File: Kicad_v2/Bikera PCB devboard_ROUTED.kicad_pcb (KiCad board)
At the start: 4 copper layers, 60 x 40 mm, 114 parts, among them IC1 DRV5032DULPGM, IC2 BQ25630YBGR, IC3 DRV5032DULPGM, IC4 FM24V01A-G, J1 USB4105-GF-A-060, J3 ST-LINK BTB, J7 Waveshare_ePaper_module, SW1 SW_Reset, SW2 SW_Boot, U1 RT6158HWSC, U2 TCR3UG33A_LF, U3 STM32L431CCTx, U4 TPS61253F, U5 ATECC608B-SSHDA-T, U6 LC76GPAMD, U7 USBLC6-2SC6, U8 SMF05CT1G, U9 RAK11720

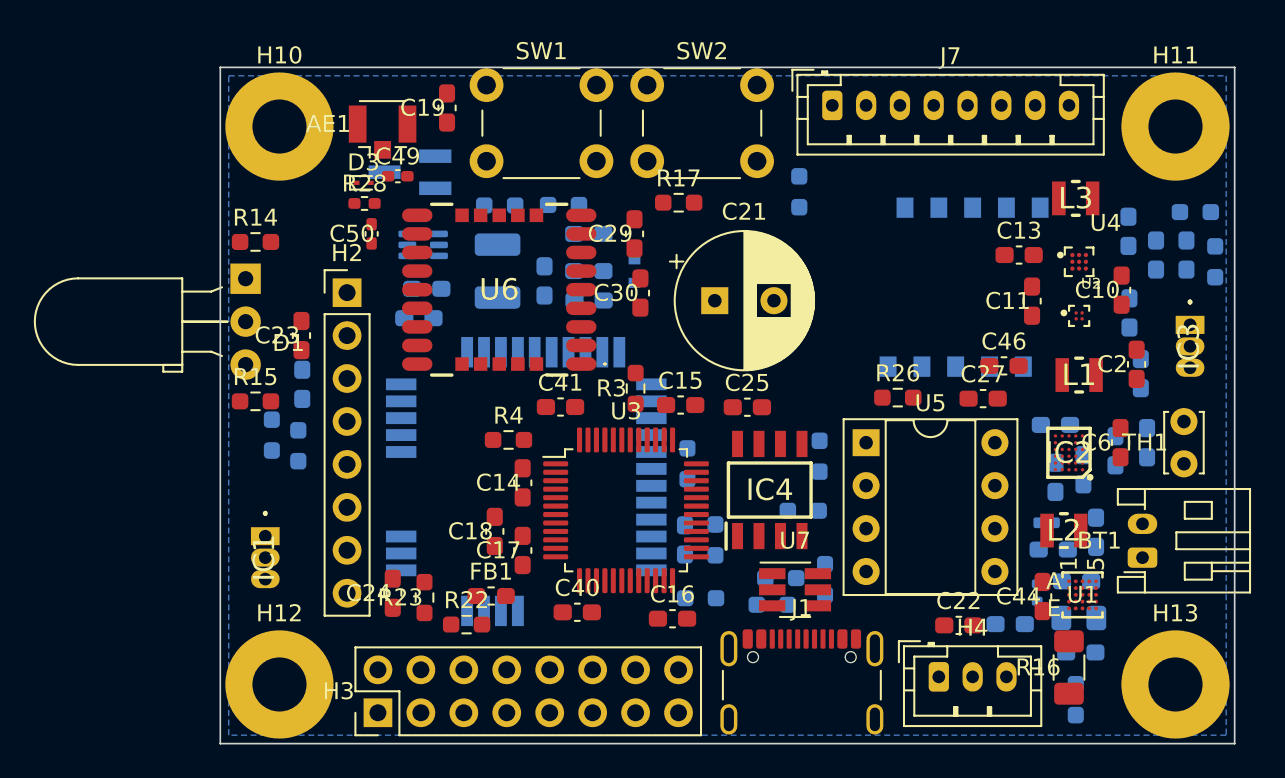
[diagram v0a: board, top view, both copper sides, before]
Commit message: PCB routing claude (deel 1)
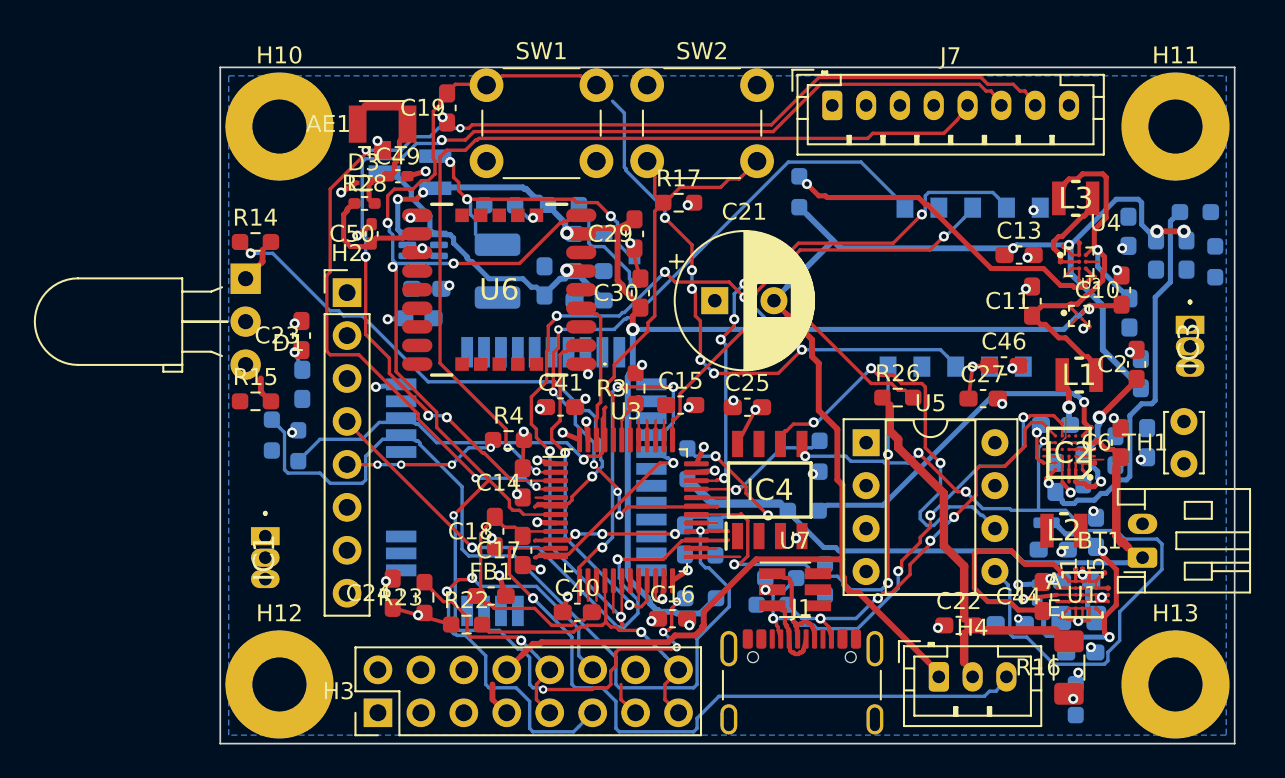
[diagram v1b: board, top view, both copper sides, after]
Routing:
- net GPS_RESET: track 0.00 -> 119.4 mm, vias 0 -> 14
- net +5V: track 0.00 -> 98.9 mm, vias 0 -> 4
- net +3V3_GPS: track 0.00 -> 78.7 mm, vias 0 -> 5
- net EPAPER_RST: track 0.00 -> 72.4 mm, vias 0 -> 4
- net EPAPER_DC: track 0.00 -> 66.1 mm, vias 0 -> 4
- net I2C_SDA: track 0.00 -> 59.0 mm, vias 0 -> 8
- net EPAPER_CS: track 0.00 -> 55.0 mm, vias 0 -> 2
- net LORA_BOOT: track 0.00 -> 53.6 mm, vias 0 -> 1
- net +SYS: track 0.00 -> 50.1 mm, vias 0 -> 2
- net /MCU - Sensors - Actuators/SERVO_RSENSE: track 0.00 -> 49.0 mm, vias 0 -> 6
- net /MCU - Sensors - Actuators/DEBUG_RX: track 0.00 -> 45.8 mm, vias 0 -> 5
- net /MCU - Sensors - Actuators/SERVO_PWM: track 0.00 -> 41.9 mm, vias 0 -> 1
- net +BATT: track 0.00 -> 39.3 mm
- net +3V3: track 0.00 -> 36.9 mm, vias 0 -> 30
- net /MCU - Sensors - Actuators/ACCEL_INT2: track 0.00 -> 35.2 mm, vias 0 -> 2
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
